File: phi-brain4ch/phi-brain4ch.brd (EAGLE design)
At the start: 76.2 x 48.3 mm, 63 parts, among them IC1 STM32F427VGT6, IC2 6N138S-TA1, IC3 AT45DB161D-SU, U1 LM1117MPX-3.3/NOPB or AP2114H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, U2 PRTR5V0U2X, U5 SN65HVD230, X2 04-JST-B4B-XH-A, X3 04-JST-B4B-XH-A, Y1 8MHz

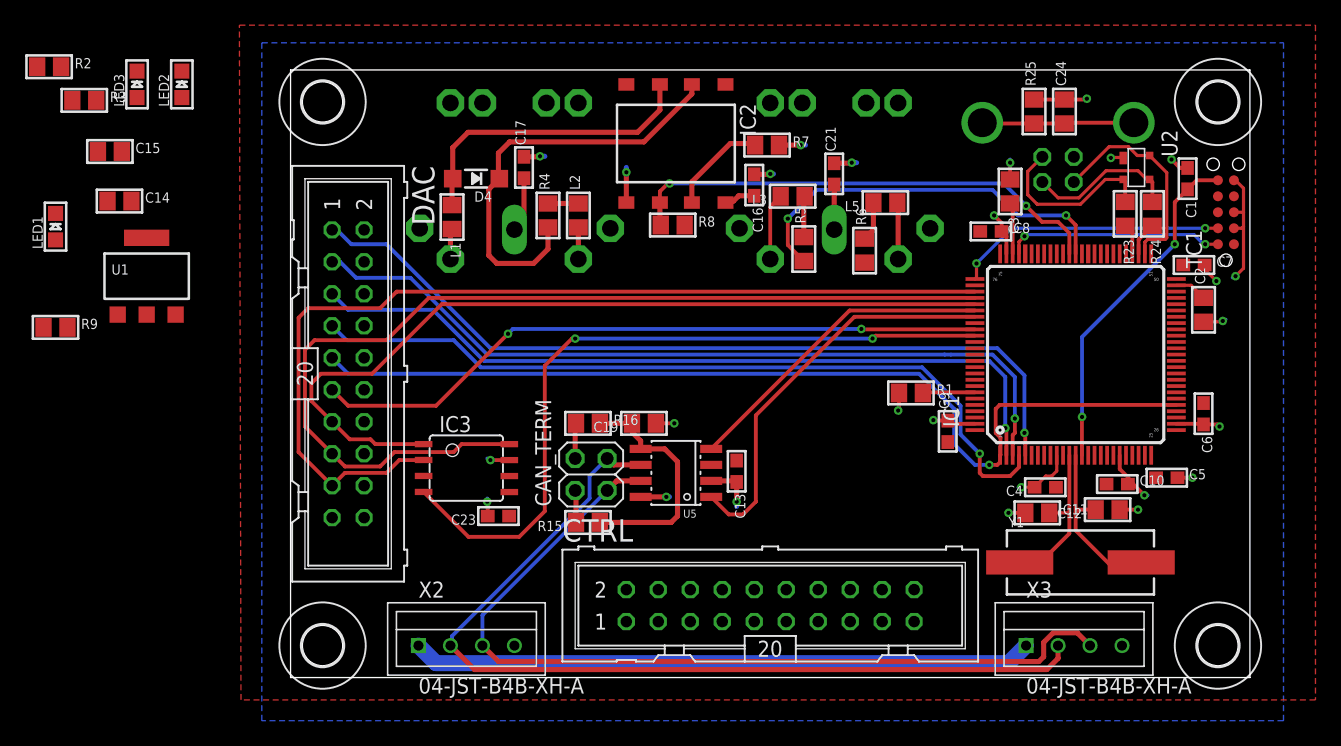
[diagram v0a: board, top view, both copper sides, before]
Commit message: wip
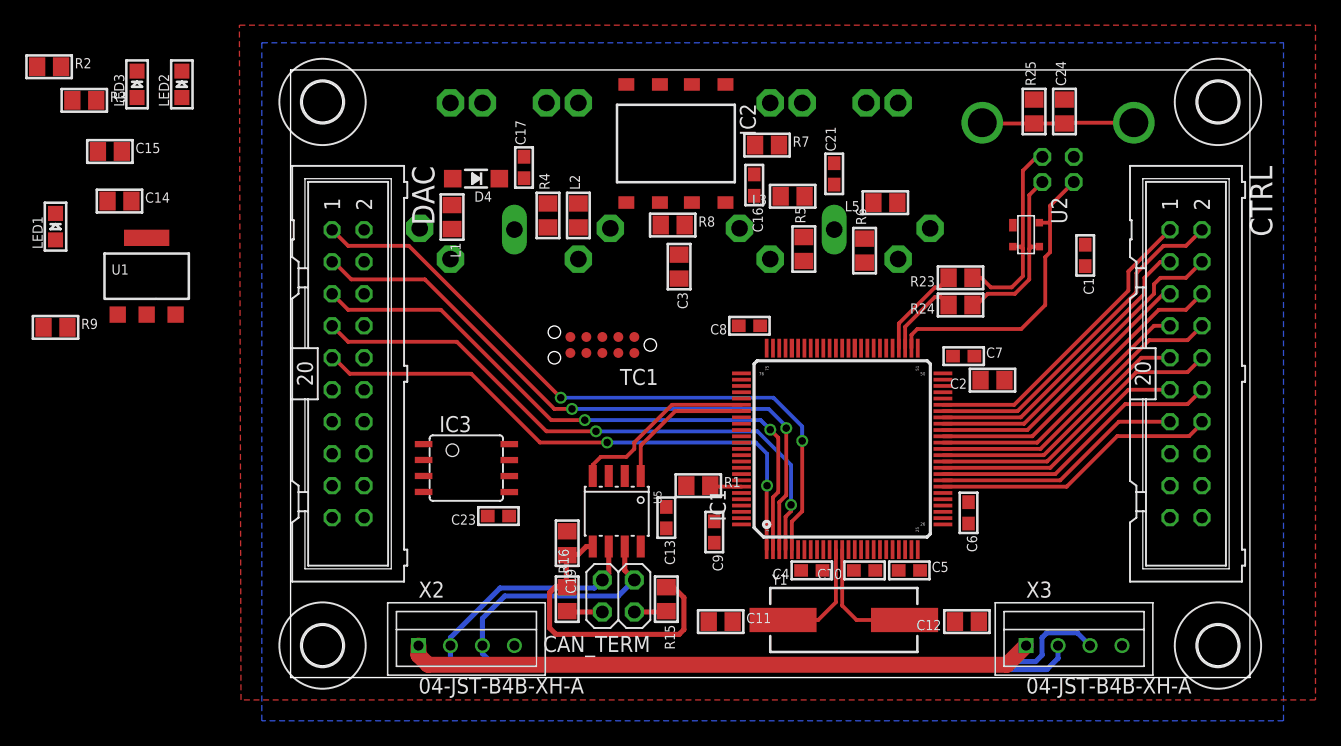
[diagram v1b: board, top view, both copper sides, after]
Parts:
- moved TC1 50.6 mm to (24.8, 26.4), turned to 180 degrees
- moved CTRL 37.8 mm to (71.1, 24.1), turned to 270 degrees
- moved C3 27.0 mm to (30.9, 32.6)
- moved C11 26.6 mm to (34.2, 4.45)
- moved C5 21.7 mm to (49.1, 8.51)
- moved C10 21.2 mm to (45.6, 8.51), turned to 180 degrees
- moved C8 20.6 mm to (36.4, 27.9), turned to 180 degrees
- moved C6 20.3 mm to (53.8, 13.1)
- moved C9 20.2 mm to (33.7, 11.6), turned to 270 degrees
- moved IC1 20.0 mm to (42.5, 16.9)
- moved C4 19.7 mm to (41.4, 8.51)
- moved C7 19.7 mm to (53.5, 25.5)
- moved Y1 19.3 mm to (43.9, 4.57)
- moved R1 18.4 mm to (32.4, 15.2)
- moved C2 17.7 mm to (55.8, 23.6), turned to 180 degrees
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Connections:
- net LCD_D2: now also IC1.40; no longer IC1.41
- net LCD_D3: now also IC1.41; no longer IC1.40
- net ROT1_A: now also IC1.32
- net ROT1_B: now also IC1.33
- net ROT1_SW: now also IC1.34
- net ROT2_A: now also IC1.36
- net ROT2_B: now also IC1.37
- net ROT2_SW: now also IC1.35
- net SPI4_MISO: now also CTRL.2; no longer CTRL.1
- net SPI4_MOSI: now also CTRL.1; no longer CTRL.2
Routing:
- net SPI3_MISO: track 79.3 -> 0.00 mm
- net SPI3_CLK: track 77.1 -> 0.00 mm
- net GND: track 69.8 -> 0.00 mm, vias 26 -> 0
- net SPI3_MOSI: track 67.0 -> 0.00 mm
- net FLASH_CS: track 58.7 -> 0.00 mm, vias 2 -> 0
- net DAC_CS: track 54.1 -> 0.00 mm, vias 2 -> 0
- net MIDI_IN: track 38.8 -> 0.00 mm, vias 2 -> 0
- net N$17: track 33.7 -> 0.00 mm
- net I2S_MCK: track 77.2 -> 45.3 mm, vias 1 -> 2
- net MIDI_OUT: track 31.1 -> 0.00 mm, vias 2 -> 0
- net SPI4_MISO: track 0.00 -> 27.4 mm
- net NRST: track 27.3 -> 0.00 mm, vias 2 -> 0
- net LCD_D4: track 0.00 -> 26.3 mm
- net LCD_D2: track 0.00 -> 25.3 mm
- net SPI4_MOSI: track 0.00 -> 24.7 mm
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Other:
- board text added: "GND AND 3.3V ARE HIDDEN"
